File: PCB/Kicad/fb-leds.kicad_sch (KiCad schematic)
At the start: 32 parts

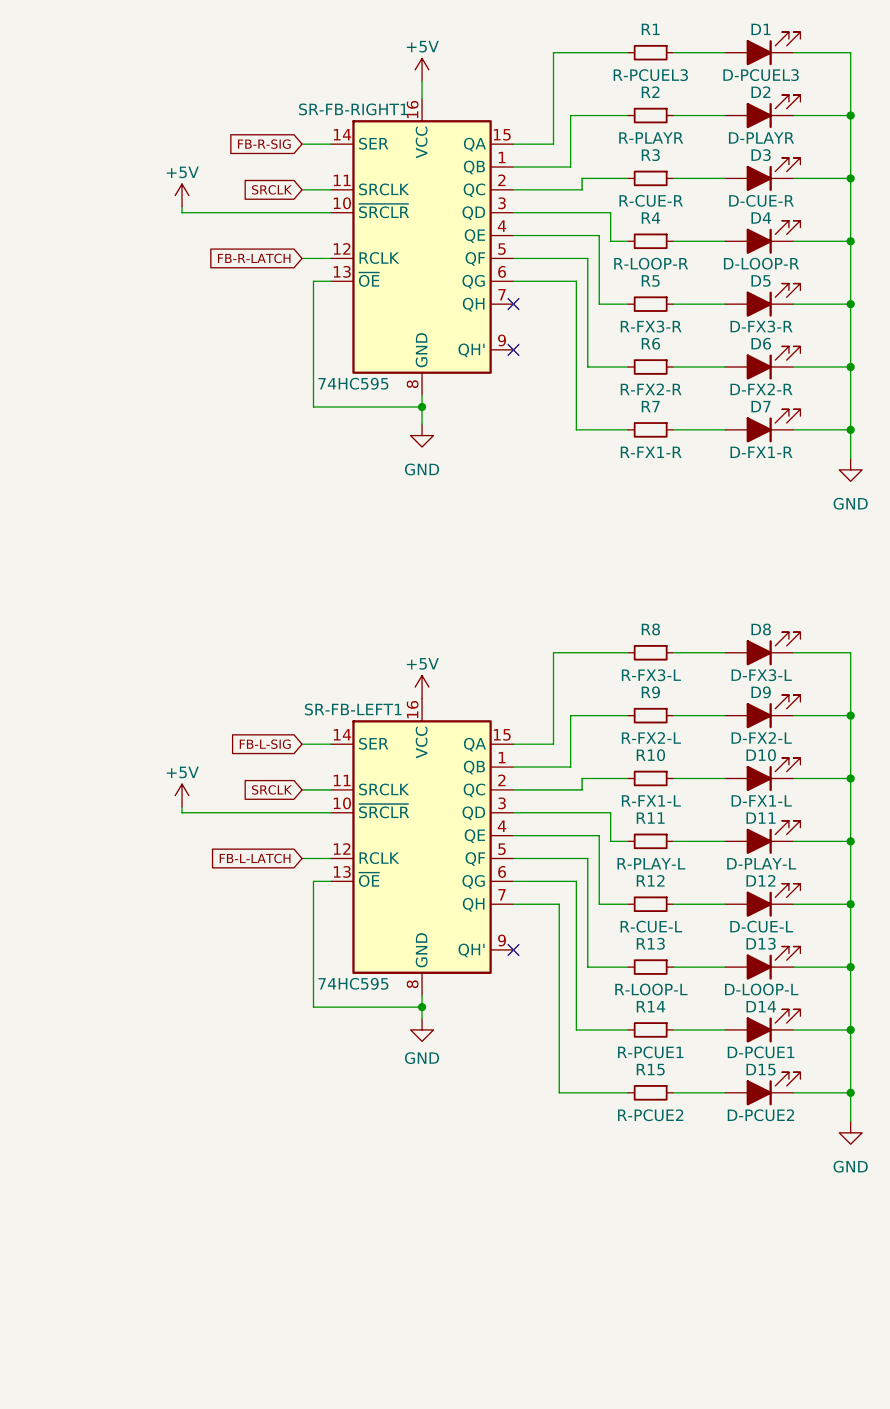
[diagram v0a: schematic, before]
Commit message: PDF
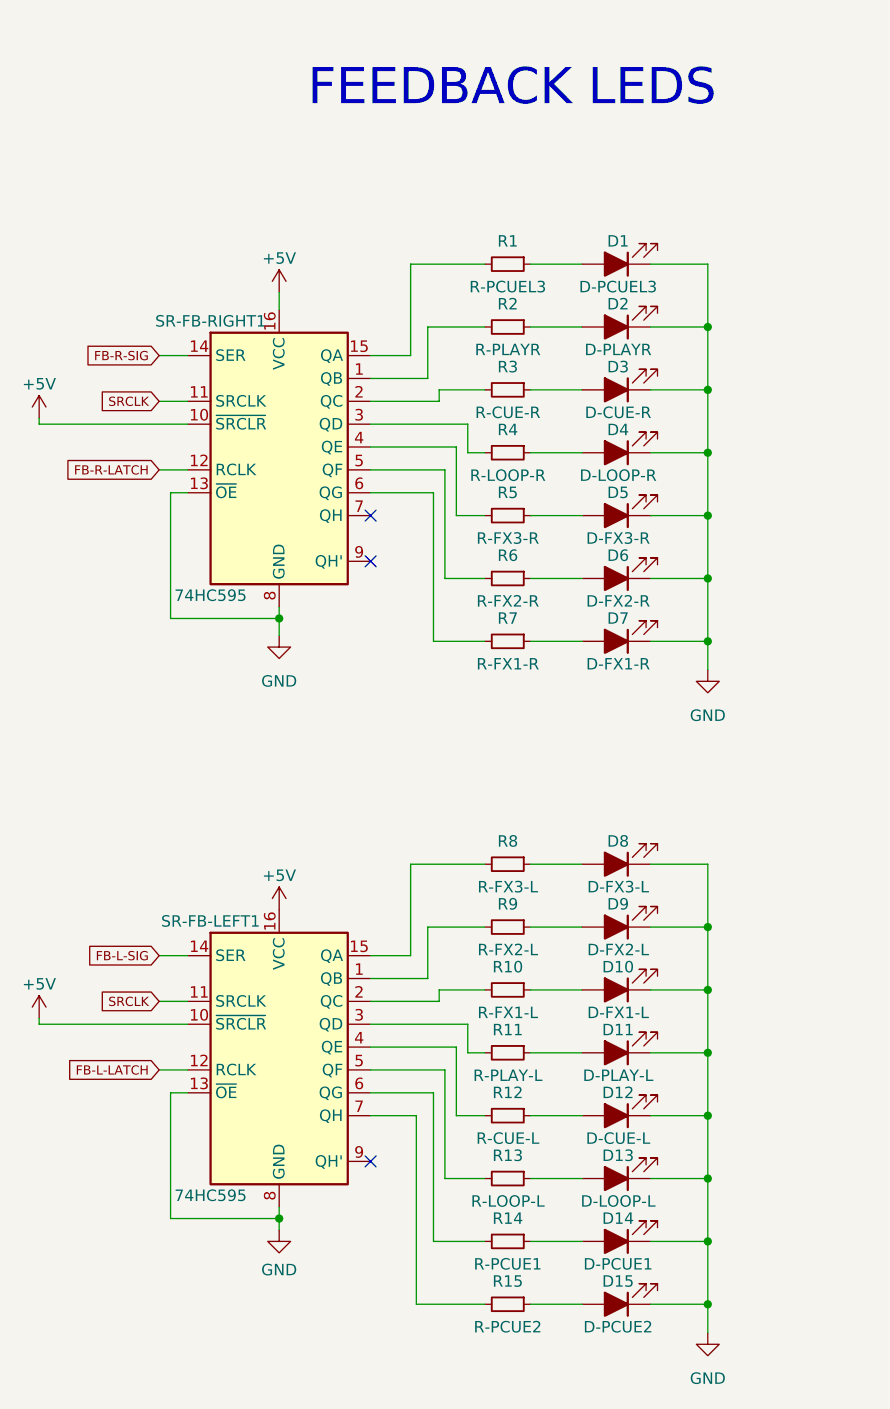
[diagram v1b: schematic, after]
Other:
- note added: "FEEDBACK LEDS"
- moved on the sheet: D1, D10, D11, D12, D13, D14, D15, D2, D3, D4, D5, D6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
